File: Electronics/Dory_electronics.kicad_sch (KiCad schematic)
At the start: 22 parts, among them J1 Bateria 2S, J10 SHARP_CENTRO_E, J4 Motor B, J5 Motor A, J6 sensor IR, J7 VL53L0X_ESQUERDO, J8 SHARP_CENTRO_D, J9 VL53L0X_DIREITO, U1 LM1117 5V

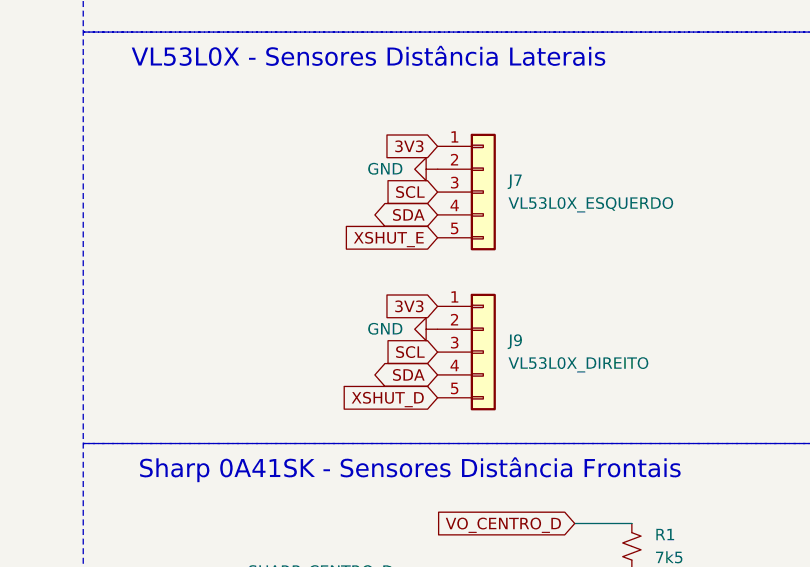
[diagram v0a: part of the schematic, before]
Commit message: chore: update PCB and create BOM file
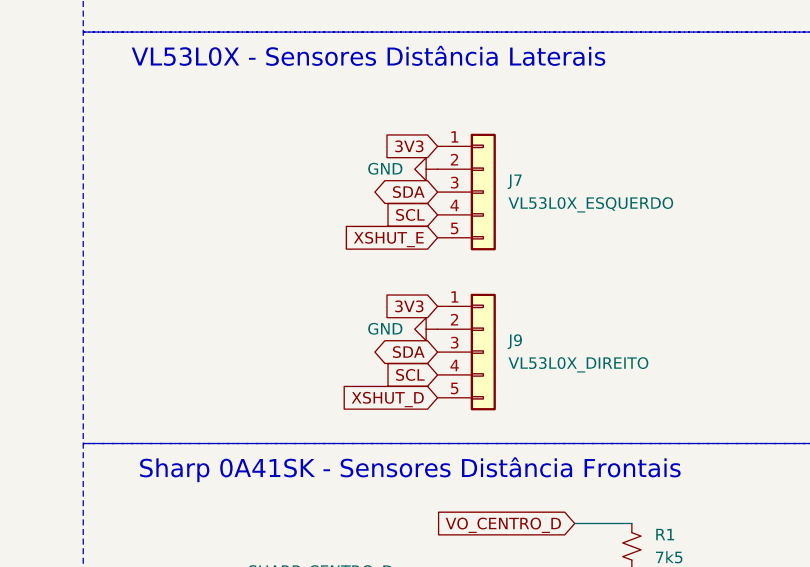
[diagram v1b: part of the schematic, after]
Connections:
- net SCL: now also J7.4 (Pin_4), J9.4 (Pin_4); no longer J7.3 (Pin_3), J9.3 (Pin_3)
- net SDA: now also J7.3 (Pin_3), J9.3 (Pin_3); no longer J7.4 (Pin_4), J9.4 (Pin_4)
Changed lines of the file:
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@@
 	(global_label "SDA"
 		(shape bidirectional)
-		(at 237.49 91.44 180)
-		(effects
-			(font
-				(size 1.27 1.27)
-			)
-			(justify right)
-		)
-		(property "Intersheetrefs" "${INTERSHEET_REFS}"
-			(at 237.49 91.44 0)
+		(at 237.49 88.9 180)
+		(effects
+			(font
+				(size 1.27 1.27)
+			)
+			(justify right)
+		)
+		(property "Intersheetrefs" "${INTERSHEET_REFS}"
+			(at 237.49 88.9 0)
 			(effects
 				(font
@@
 	(global_label "SDA"
 		(shape bidirectional)
-		(at 237.49 73.66 180)
-		(effects
-			(font
-				(size 1.27 1.27)
-			)
-			(justify right)
-		)
-		(property "Intersheetrefs" "${INTERSHEET_REFS}"
-			(at 237.49 73.66 0)
+		(at 237.49 71.12 180)
+		(effects
+			(font
+				(size 1.27 1.27)
+			)
+			(justify right)
+		)
+		(property "Intersheetrefs" "${INTERSHEET_REFS}"
+			(at 237.49 71.12 0)
 			(effects
 				(font
@@
 	(global_label "SCL"
 		(shape input)
-		(at 237.49 88.9 180)
-		(effects
-			(font
-				(size 1.27 1.27)
-			)
-			(justify right)
-		)
-		(property "Intersheetrefs" "${INTERSHEET_REFS}"
-			(at 237.49 88.9 0)
+		(at 237.49 91.44 180)
+		(effects
+			(font
+				(size 1.27 1.27)
+			)
+			(justify right)
+		)
+		(property "Intersheetrefs" "${INTERSHEET_REFS}"
+			(at 237.49 91.44 0)
 			(effects
 				(font
@@
 	(global_label "SCL"
 		(shape input)
-		(at 237.49 71.12 180)
-		(effects
-			(font
-				(size 1.27 1.27)
-			)
-			(justify right)
-		)
-		(property "Intersheetrefs" "${INTERSHEET_REFS}"
-			(at 237.49 71.12 0)
-			(effects
-				(font
+		(at 237.49 73.66 180)
+		(effects
+			(font
+				(size 1.27 1.27)
+			)
+			(justify right)
+		)
+		(property "Intersheetrefs" "${INTERSHEET_REFS}"
+			(at 237.49 73.66 0)
+			(effects
+				(font
